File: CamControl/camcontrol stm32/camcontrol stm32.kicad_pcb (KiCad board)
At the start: 4 copper layers, 15.9 x 33.8 mm, 54 parts, among them J1 Power 1, J2 Conn_01x04, J3 Power 1, J4 Power 1, J5 Conn_01x06, J6 Conn_01x02, J7 Power 1, Q1 AO3401A, U1 BGS12P2L6, U2 BALFHB-WL-02D3, U3 STM32WLE4CCUx, U4 DS8242, U5 TPS25970LRPWR, U6 TPS25970LRPWR, U7 INA2180, Y1 32MHz

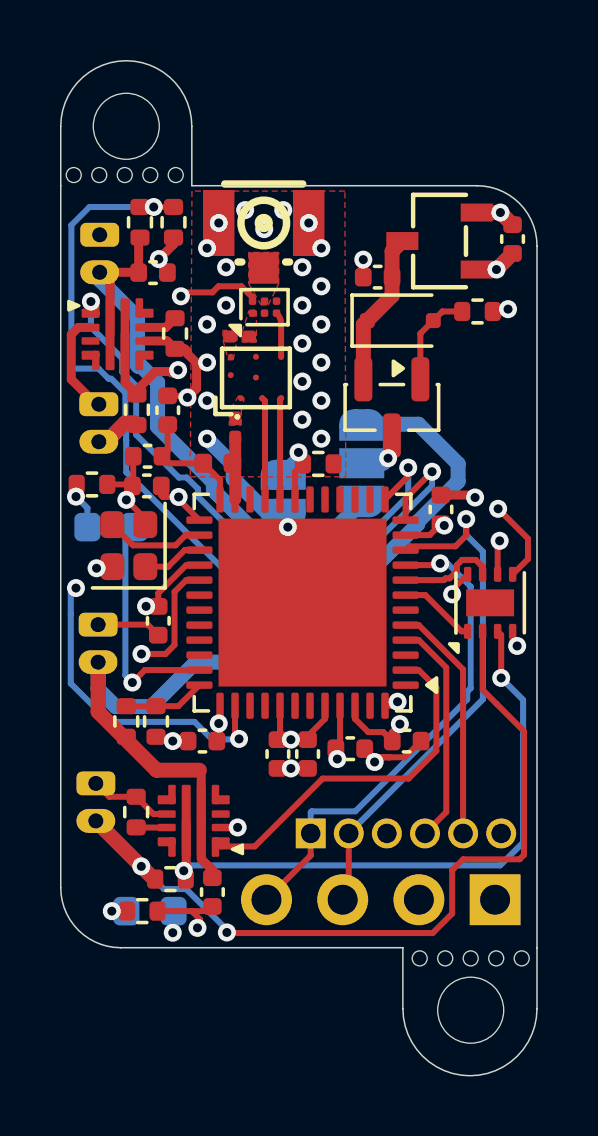
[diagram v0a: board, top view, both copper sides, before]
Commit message: shit make it good
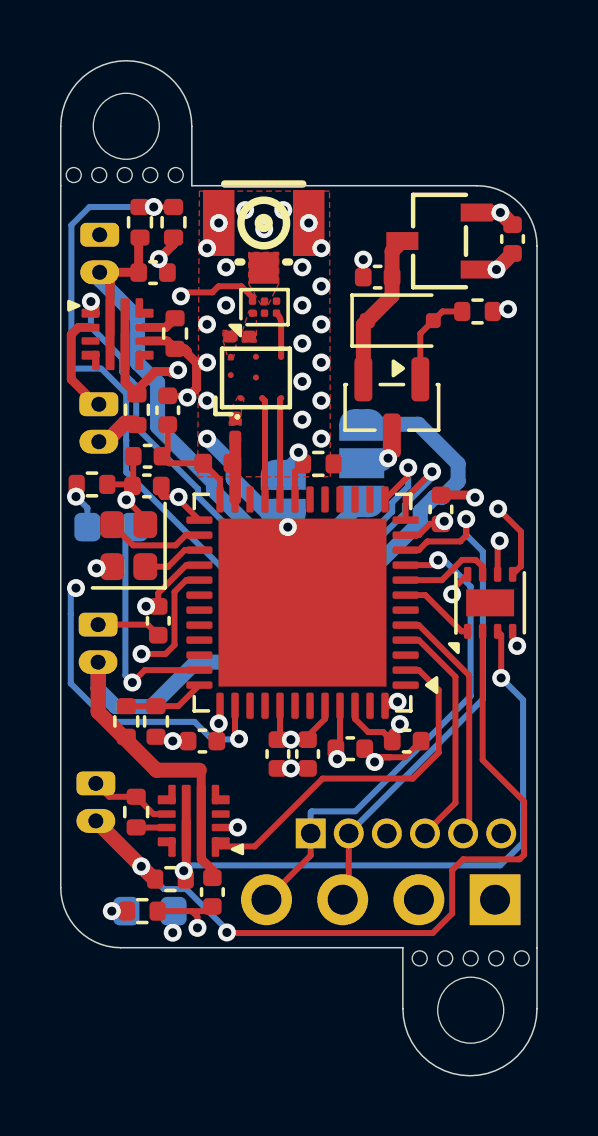
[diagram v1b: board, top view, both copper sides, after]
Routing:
- net +3V3: track 22.2 -> 16.4 mm
- net /PWR B SENS: track 26.3 -> 25.1 mm
